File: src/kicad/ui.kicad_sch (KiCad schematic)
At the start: 11 parts, among them SW1 RotaryEncoder_Switch, SW10 SW_Push, SW2 SW_Slide_DPDT, SW3 SW_Push, SW4 SW_Push, SW5 SW_Push, SW6 SW_Push, SW7 SW_Push, SW8 SW_Push, SW9 SW_Push

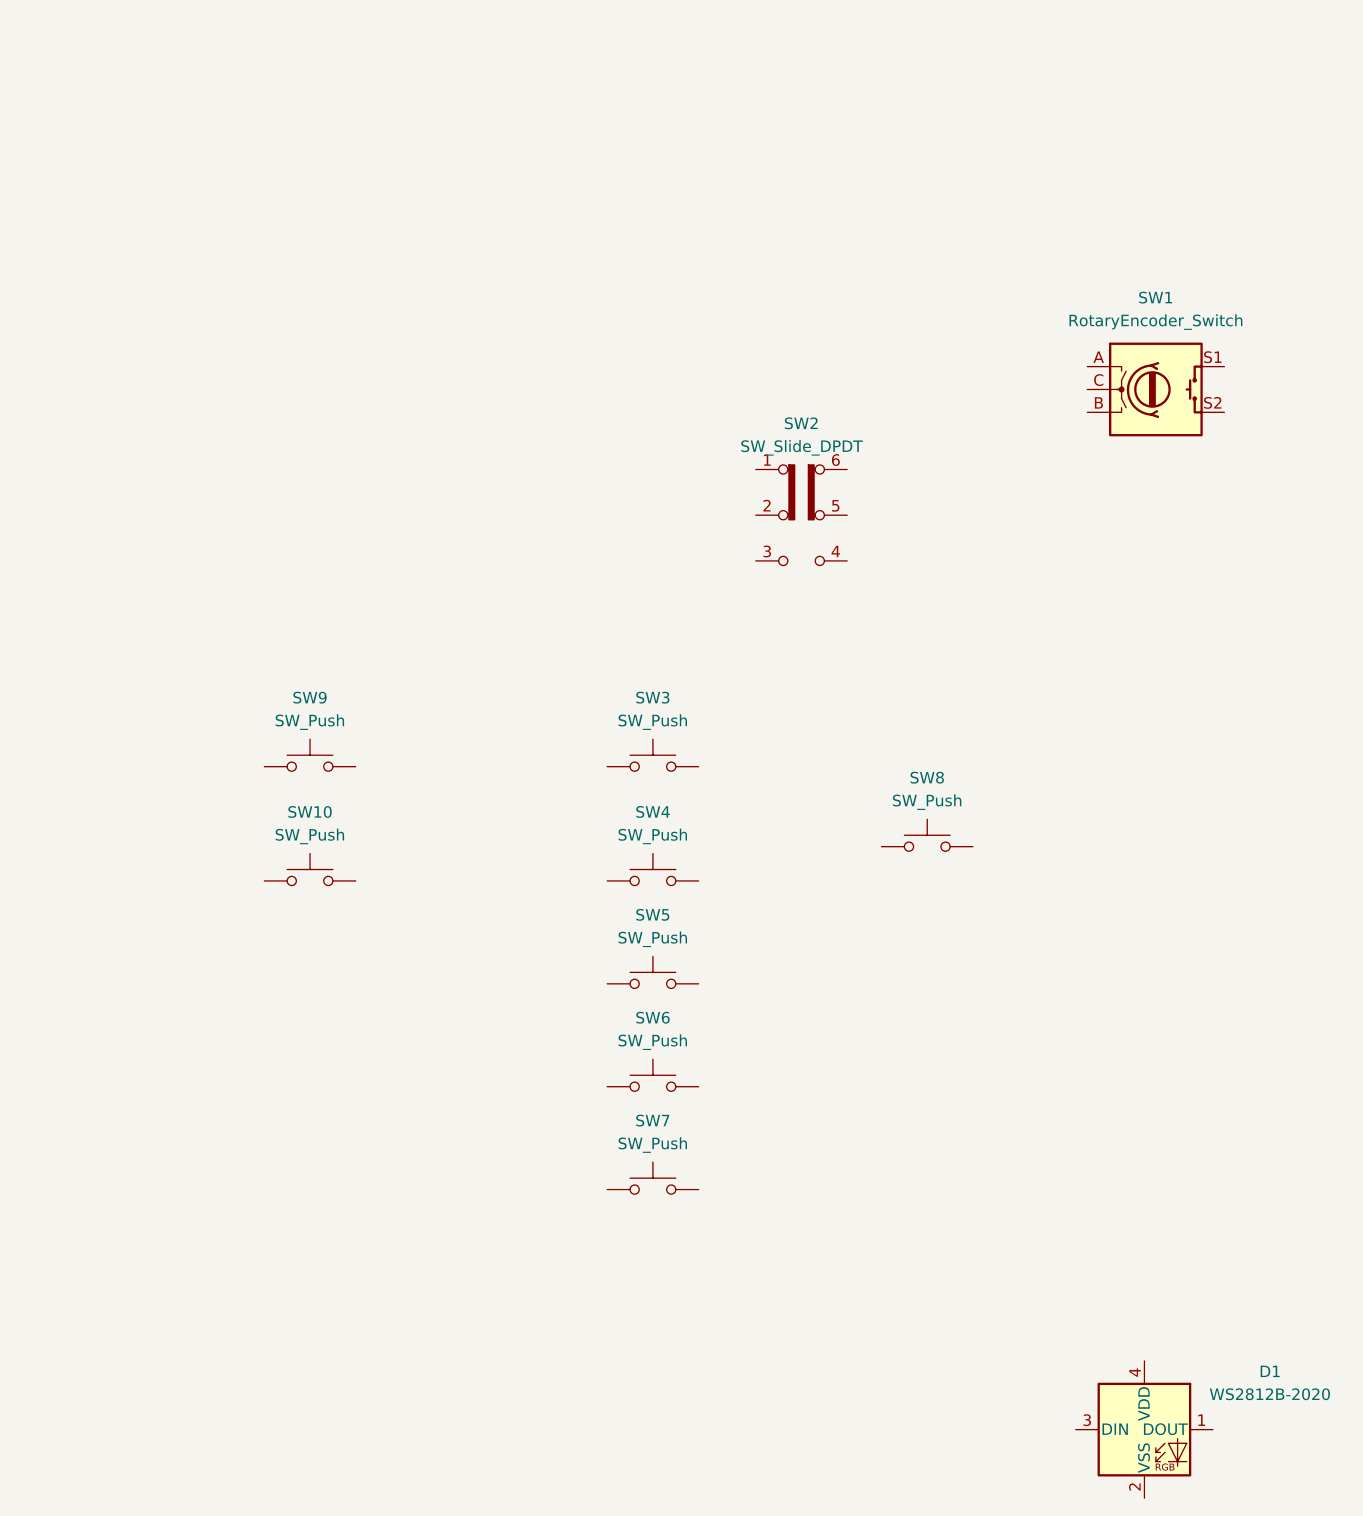
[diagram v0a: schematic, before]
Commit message: progress + new journal entry!
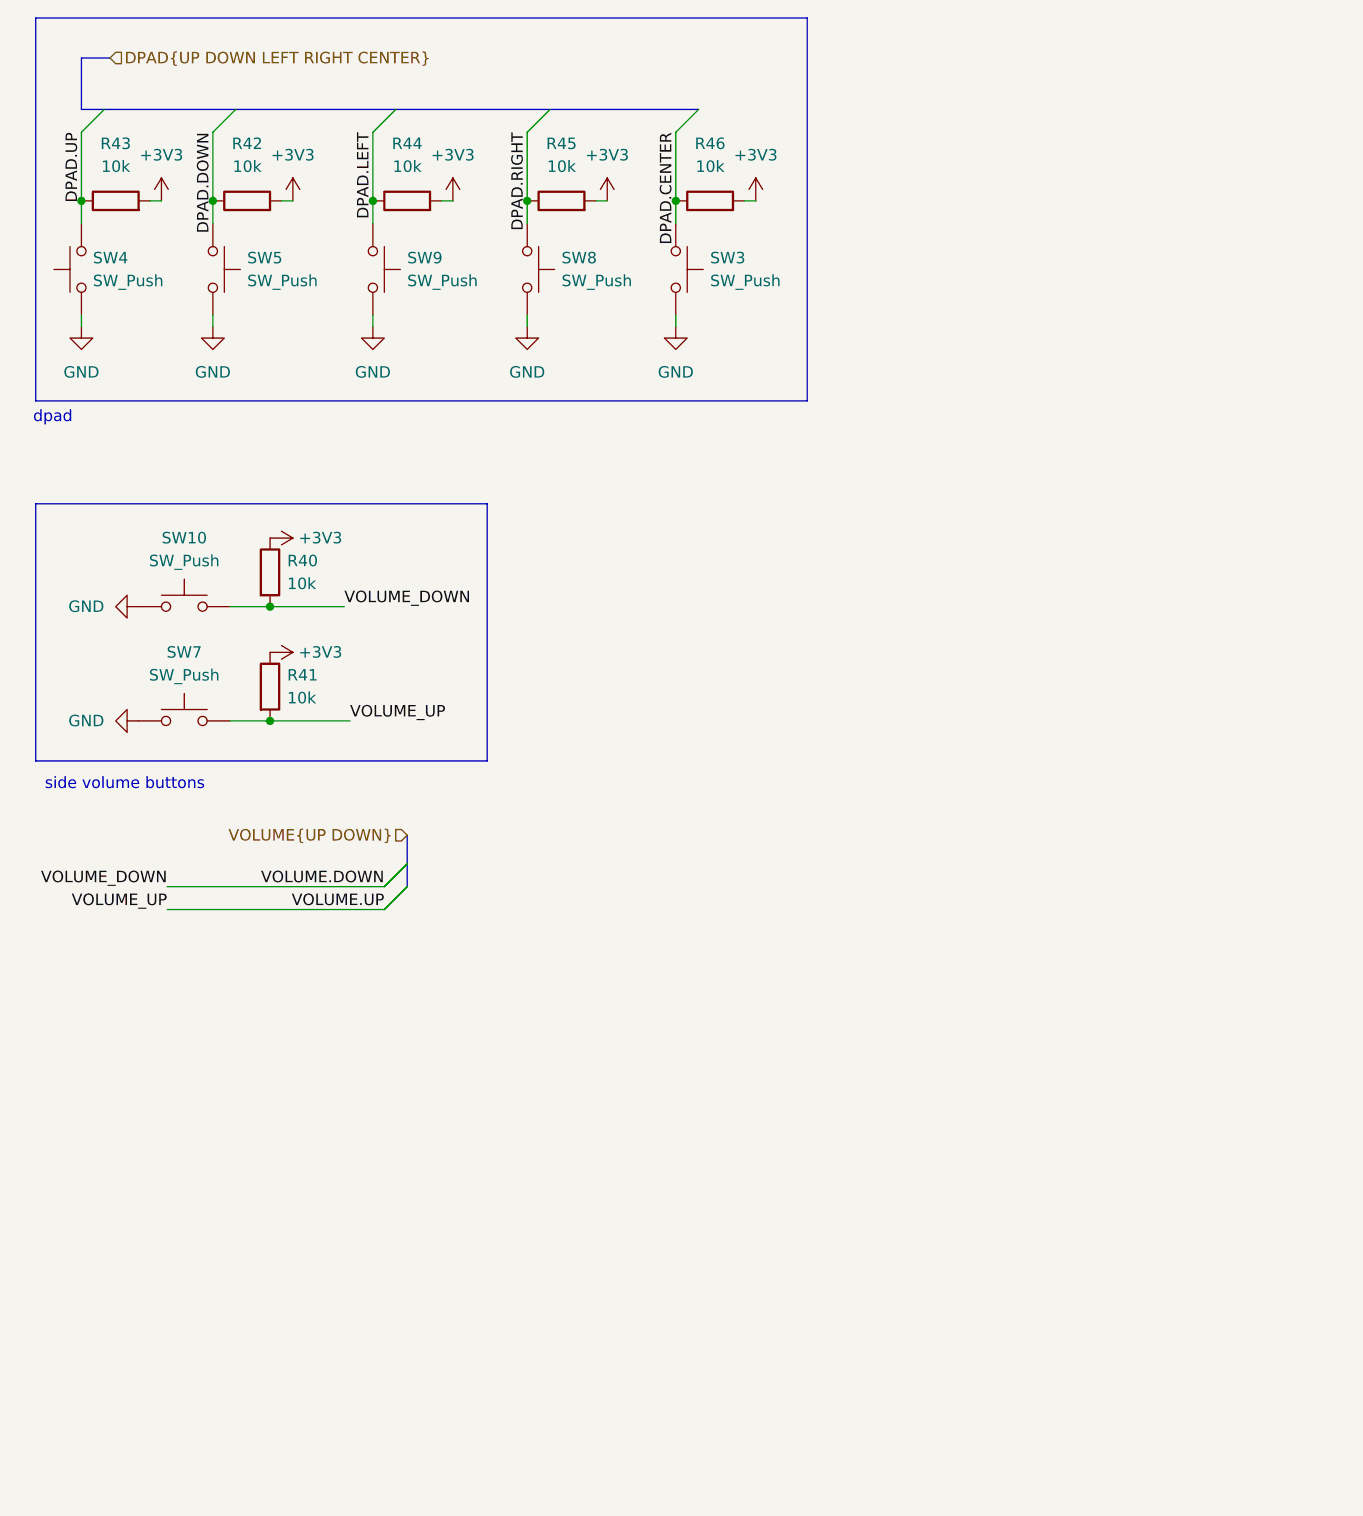
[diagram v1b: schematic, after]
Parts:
- removed D1: WS2812B-2020, LED_SMD:LED_WS2812B-2020_PLCC4_2.0x2.0mm, symbol LED:WS2812B-2020
- removed SW1: RotaryEncoder_Switch, symbol Device:RotaryEncoder_Switch
- removed SW2: SW_Slide_DPDT, symbol Switch:SW_Slide_DPDT
- removed SW6: SW_Push, symbol Switch:SW_Push
- added R40, R41, R42, R43, R44, R45, R46: 10k, symbol Device:R
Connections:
- net GND: now reaches SW7.1
- net GND: now also SW10.1, SW3.2, SW4.1, SW5.2, SW8.2, SW9.2
- net VOLUME.UP: now reaches SW7.2
- net VOLUME.UP: now also R41.2
- net DPAD.RIGHT: now reaches SW8.1
- net DPAD.RIGHT: now also R45.1
- net DPAD.LEFT: now reaches SW9.1
- net DPAD.LEFT: now also R44.1
- net DPAD.UP: now reaches SW4.2
- net DPAD.UP: now also R43.1
- net DPAD.CENTER: now reaches SW3.1
- net DPAD.CENTER: now also R46.1
- net DPAD.DOWN: now reaches SW5.1
- net DPAD.DOWN: now also R42.1
- net VOLUME.DOWN: now reaches SW10.2
- net VOLUME.DOWN: now also R40.2
- new net +3V3: R40.1, R41.1, R42.2, R43.2, R44.2, R45.2, R46.2
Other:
- note added: "dpad"
- note added: "side volume buttons"
- moved on the sheet: SW10, SW3, SW4, SW5, SW7, SW8, SW9

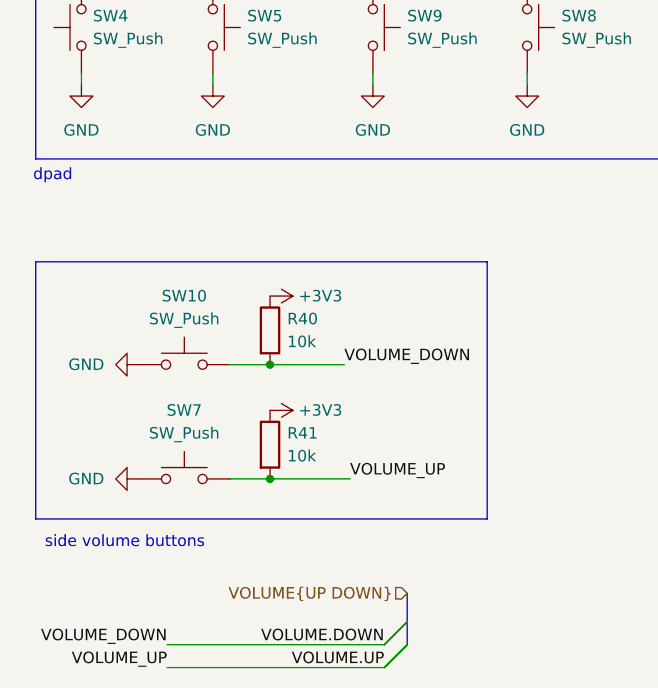
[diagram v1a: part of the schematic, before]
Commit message: may 28th
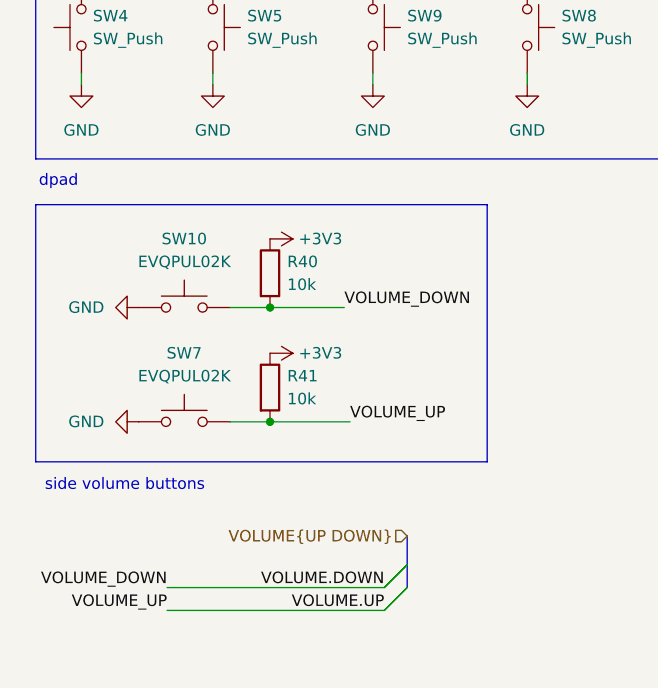
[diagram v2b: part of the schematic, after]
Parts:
- R40, R41, R42, R43, R44, R45, R46: footprint (none) -> Resistor_SMD:R_0402_1005Metric
- SW10, SW7: value SW_Push -> EVQPUL02K; footprint (none) -> EVQPUL02K:KEY-SMD_4P-L4.7-W3.5-P1.70-LS6.4-EH; LCSC Part (none) -> C79175
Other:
- moved on the sheet: R40, R41, SW10, SW7

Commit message: more components associations
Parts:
- R40, R41, R42, R43, R44, R45, R46: LCSC Part (none) -> C25744
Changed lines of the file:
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@@
+			)
+		)
+		(property "LCSC Part" "C25744"
+			(at 25.4 36.195 90)
+			(hide yes)
+			(show_name no)
+			(do_not_autoplace no)
+			(effects
+				(font
+					(size 1.27 1.27)
+				)
 			)
 		)
@@
 			)
 		)
+		(property "LCSC Part" "C25744"
+			(at 91.44 36.195 90)
+			(hide yes)
+			(show_name no)
+			(do_not_autoplace no)
+			(effects
+				(font
+					(size 1.27 1.27)
+				)
+			)
+		)
 		(pin "2"
 		)
@@
 			)
 		)
+		(property "LCSC Part" "C25744"
+			(at 42.545 71.12 0)
+			(hide yes)
+			(show_name no)
+			(do_not_autoplace no)
+			(effects
+				(font
+					(size 1.27 1.27)
+				)
+			)
+		)
 		(pin "2"
 		)
@@
 			)
 		)
+		(property "LCSC Part" "C25744"
+			(at 57.785 36.195 90)
+			(hide yes)
+			(show_name no)
+			(do_not_autoplace no)
+			(effects
+				(font
+					(size 1.27 1.27)
+				)
+			)
+		)
 		(pin "2"
 		)
@@
 			)
 		)
+		(property "LCSC Part" "C25744"
+			(at 40.005 36.195 90)
+			(hide yes)
+			(show_name no)
+			(do_not_autoplace no)
+			(effects
+				(font
+					(size 1.27 1.27)
+				)
+			)
+		)
 		(pin "2"
 		)
@@
 			)
 		)
+		(property "LCSC Part" "C25744"
+			(at 42.545 83.82 0)
+			(hide yes)
+			(show_name no)
+			(do_not_autoplace no)
+			(effects
+				(font
+					(size 1.27 1.27)
+				)
+			)
+		)
 		(pin "2"
 		)
@@
 			(at 74.93 36.195 90)
 			(hide yes)
+			(show_name no)
+			(do_not_autoplace no)
+			(effects
+				(font
+					(size 1.27 1.27)
+				)
+			)
+		)
+		(property "LCSC Part" "C25744"
+			(at 74.93 36.195 90)
+			(hide yes)

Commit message: may 29th + files updates
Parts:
- SW3, SW4, SW5, SW8, SW9: footprint (none) -> easyeda2kicad:SW-SMD_4P-L6.2-W6.2-P4.00-LS6.8; LCSC Part (none) -> C115354
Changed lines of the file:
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@@
 			)
 		)
-		(property "Footprint" ""
+		(property "Footprint" "easyeda2kicad:SW-SMD_4P-L6.2-W6.2-P4.00-LS6.8"
 			(at 76.2 43.815 0)
 			(hide yes)
@@
 		)
 		(property "KLC_S4.2_VREG_LX" ""
+			(at 71.12 43.815 90)
+			(hide yes)
+			(show_name no)
+			(do_not_autoplace no)
+			(effects
+				(font
+					(size 1.27 1.27)
+				)
+			)
+		)
+		(property "LCSC Part" "C115354"
 			(at 71.12 43.815 90)
 			(hide yes)
@@
 			)
 		)
-		(property "Footprint" ""
+		(property "Footprint" "easyeda2kicad:SW-SMD_4P-L6.2-W6.2-P4.00-LS6.8"
 			(at 59.055 43.815 0)
 			(hide yes)
@@
 		)
 		(property "KLC_S4.2_VREG_LX" ""
+			(at 53.975 43.815 90)
+			(hide yes)
+			(show_name no)
+			(do_not_autoplace no)
+			(effects
+				(font
+					(size 1.27 1.27)
+				)
+			)
+		)
+		(property "LCSC Part" "C115354"
 			(at 53.975 43.815 90)
 			(hide yes)
@@
 			)
 		)
-		(property "Footprint" ""
+		(property "Footprint" "easyeda2kicad:SW-SMD_4P-L6.2-W6.2-P4.00-LS6.8"
 			(at 16.51 43.815 0)
 			(hide yes)
@@
 		)
 		(property "KLC_S4.2_VREG_LX" ""
+			(at 21.59 43.815 90)
+			(hide yes)
+			(show_name no)
+			(do_not_autoplace no)
+			(effects
+				(font
+					(size 1.27 1.27)
+				)
+			)
+		)
+		(property "LCSC Part" "C115354"
 			(at 21.59 43.815 90)
 			(hide yes)
@@
 			)
 		)
-		(property "Footprint" ""
+		(property "Footprint" "easyeda2kicad:SW-SMD_4P-L6.2-W6.2-P4.00-LS6.8"
 			(at 92.71 43.815 0)
 			(hide yes)
@@
 		)
 		(property "KLC_S4.2_VREG_LX" ""
+			(at 87.63 43.815 90)
+			(hide yes)
+			(show_name no)
+			(do_not_autoplace no)
+			(effects
+				(font
+					(size 1.27 1.27)
+				)
+			)
+		)
+		(property "LCSC Part" "C115354"
 			(at 87.63 43.815 90)
 			(hide yes)
@@
 			)
 		)
-		(property "Footprint" ""
+		(property "Footprint" "easyeda2kicad:SW-SMD_4P-L6.2-W6.2-P4.00-LS6.8"
 			(at 41.275 43.815 0)
 			(hide yes)
@@
 			(at 36.195 43.815 90)
 			(hide yes)
+			(show_name no)
+			(do_not_autoplace no)
+			(effects
+				(font
+					(size 1.27 1.27)
+				)
+			)
+		)
+		(property "LCSC Part" "C115354"
+			(at 36.195 43.815 90)
+			(hide yes)

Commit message: routing + may 30th update + things
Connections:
- net GND: now also SW10.2; no longer SW10.1
- net VOLUME.DOWN: now also SW10.1; no longer SW10.2
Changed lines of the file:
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@@
 		(lib_id "Switch:SW_Push")
 		(at 33.02 74.93 0)
+		(mirror y)
 		(unit 1)
 		(body_style 1)
@@
 		(in_pos_files yes)
 		(dnp no)
-		(fields_autoplaced yes)
 		(property "Reference" "SW10"
 			(at 33.02 67.31 0)

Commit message: cad added + journal/bom update
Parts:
- R40, R41, R42, R43, R44, R45, R46: LCSC Part C25744 -> C2906861
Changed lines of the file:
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@@
 			)
 		)
-		(property "LCSC Part" "C25744"
+		(property "LCSC Part" "C2906861"
 			(at 25.4 36.195 90)
 			(hide yes)
@@
 			)
 		)
-		(property "LCSC Part" "C25744"
+		(property "LCSC Part" "C2906861"
 			(at 91.44 36.195 90)
 			(hide yes)
@@
 			)
 		)
-		(property "LCSC Part" "C25744"
+		(property "LCSC Part" "C2906861"
 			(at 42.545 71.12 0)
 			(hide yes)
@@
 			)
 		)
-		(property "LCSC Part" "C25744"
+		(property "LCSC Part" "C2906861"
 			(at 57.785 36.195 90)
 			(hide yes)
@@
 			)
 		)
-		(property "LCSC Part" "C25744"
+		(property "LCSC Part" "C2906861"
 			(at 40.005 36.195 90)
 			(hide yes)
@@
 			)
 		)
-		(property "LCSC Part" "C25744"
+		(property "LCSC Part" "C2906861"
 			(at 42.545 83.82 0)
 			(hide yes)
@@
 			)
 		)
-		(property "LCSC Part" "C25744"
+		(property "LCSC Part" "C2906861"
 			(at 74.93 36.195 90)
 			(hide yes)
